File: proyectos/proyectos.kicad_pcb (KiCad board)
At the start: 2 copper layers, 55.9 x 30.2 mm, 54 parts, among them P1 CONN_01X02, P2 CONN_01X03, P3 CONN_01X05, P4 CONN_01X03, P5 CONN_01X03, P6 CONN_01X02, U1 AD8232_A, U2 ADP3303-3.3, U3 PIC16F688, Y1 Crystal_8MHz

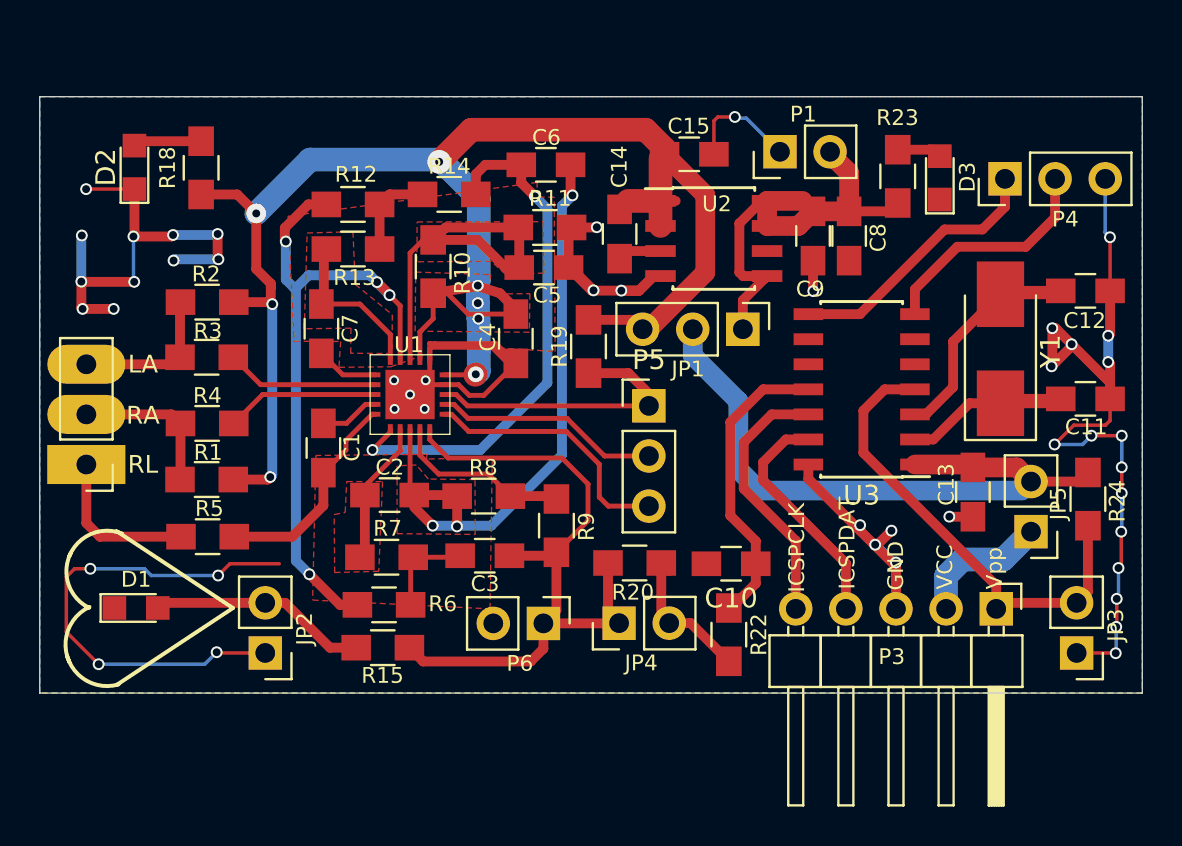
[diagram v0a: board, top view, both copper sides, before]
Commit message: VERSION 1.7 ECG Y PIC
NUEVA VERSION
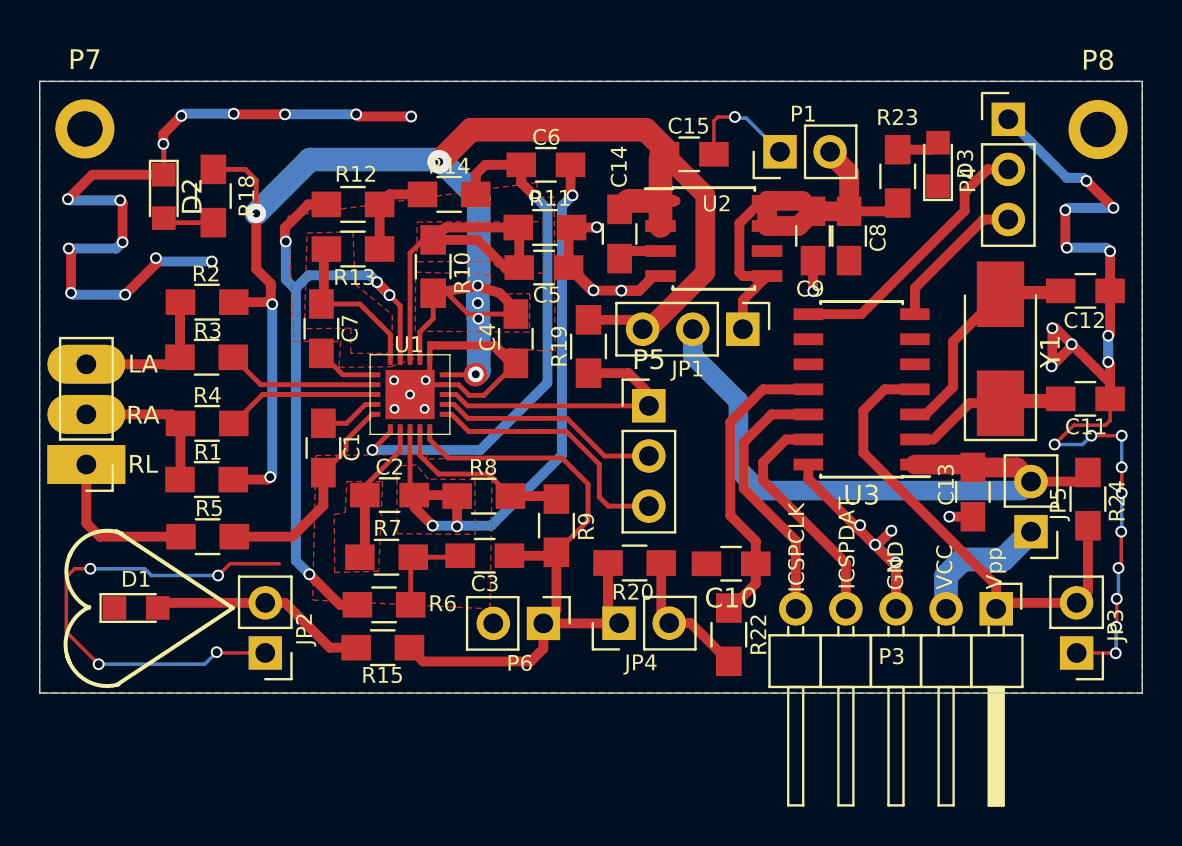
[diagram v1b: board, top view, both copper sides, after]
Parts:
- added P7: CONN_01X01, Huellas:MountingHole_1.8mm_Pad, F.Cu at (119.9, 86.6)
- added P8: CONN_01X01, Huellas:MountingHole_1.8mm_Pad, F.Cu at (171.2, 86.6)
- moved P4 3.02 mm to (166.7, 86.1), turned to 0 degrees
- moved D2 2.09 mm to (123.9, 90.0), turned to 270 degrees
- moved R18 1.56 mm to (126.4, 90.0), turned to 270 degrees
- moved D3 0.69 mm to (163.1, 88.4)
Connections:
- P4 pad 1: /O_DIG1 -> /GND
- P4 pad 2: /O_DIG2 -> /O_DIG1
- P4 pad 3: /GND -> /O_DIG2
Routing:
- net /GND: track 150.3 -> 175.9 mm, vias 46 -> 53
- net /O_DIG2: track 11.8 -> 7.50 mm
- net +vs: track 92.2 -> 93.1 mm
- net Net-(D2-Pad2): track 3.47 -> 2.61 mm
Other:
- board size 55.9 x 30.2 mm -> 55.9 x 31 mm
